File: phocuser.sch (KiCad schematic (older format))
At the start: 44 parts, among them J1 Conn_01x04_Male, J2 Conn_ARM_JTAG_SWD_10, J3 Conn_01x02_Male, J4 DX07S016JA1R1500, J5 Accessory 0, J6 Accessory 1, U1 HolyIot-18010, U2 TMC2130-LA, U3 FT231XQ

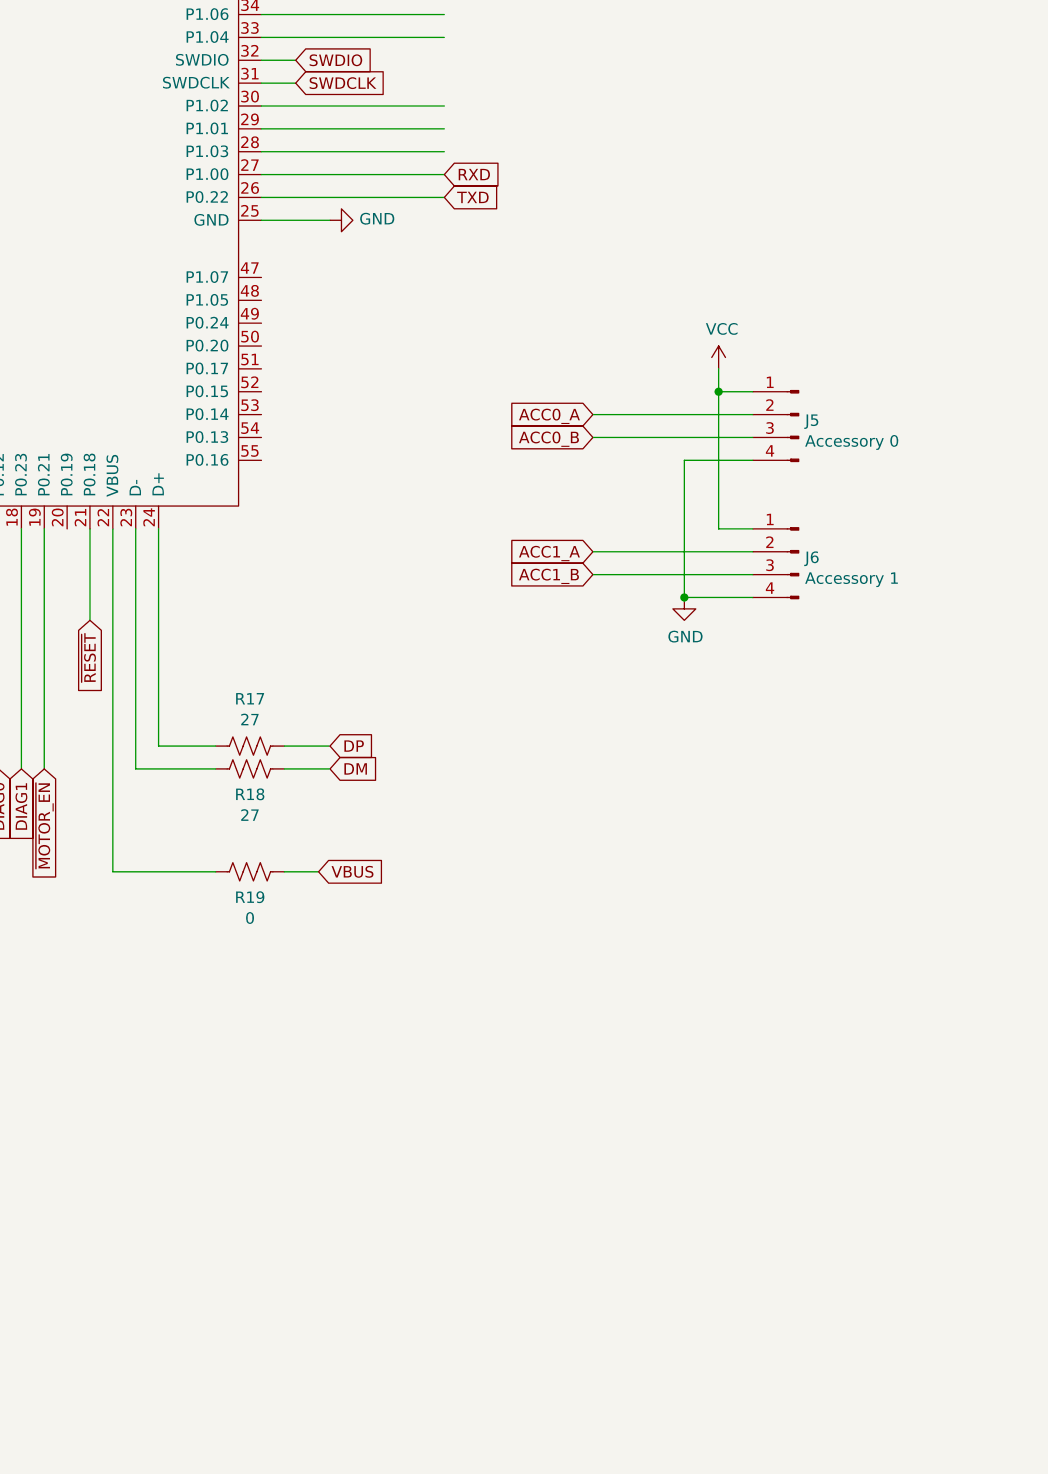
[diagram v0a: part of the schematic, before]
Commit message: layout complete
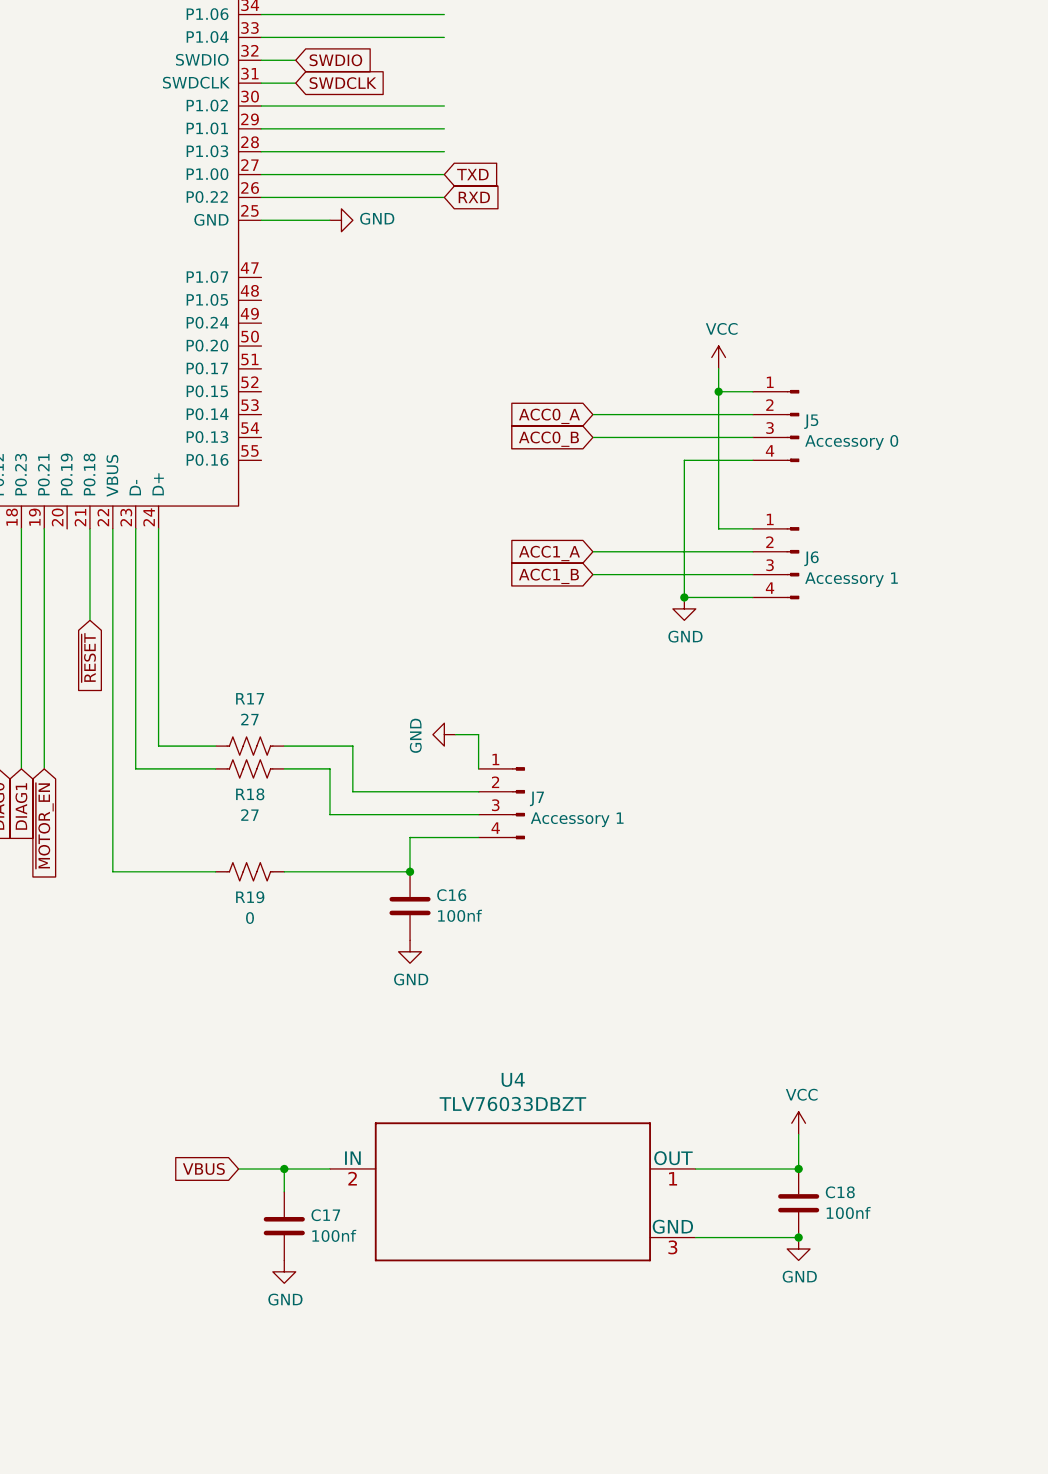
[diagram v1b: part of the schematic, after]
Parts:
- added C16, C17, C18: 100nf, Capacitor_SMD:C_0402_1005Metric, symbol Device:C
- added J7: Accessory 1, Connector_JST:JST_PH_B4B-PH-K_1x04_P2.00mm_Vertical, symbol Connector:Conn_01x04_Male
- added U4: TLV76033DBZT, footprints:TLV76033DBZT, symbol 2021-02-23_16-41-07:TLV76033DBZT
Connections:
- wire segments 191 -> 205
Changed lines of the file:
@@
 Wire Wire Line
 	4450 9450 4450 9600
+Text GLabel 6600 2400 2    50   Input ~ 0
+TXD
 Text GLabel 6600 2500 2    50   Input ~ 0
-TXD
-Text GLabel 6600 2400 2    50   Input ~ 0
 RXD
 $Comp
@@
 	0    1    1    0
 $EndComp
-Text GLabel 6100 4900 2    50   Input ~ 0
-DP
-Text GLabel 6100 5000 2    50   Input ~ 0
-DM
 Wire Wire Line
 	5350 3950 5350 4900
 Wire Wire Line
 	5350 4900 5600 4900
-Wire Wire Line
-	5900 4900 6100 4900
 Wire Wire Line
 	6100 5000 5900 5000
@@
 Wire Wire Line
 	5150 5450 5150 3950
-Text GLabel 6050 5450 2    50   Input ~ 0
-VBUS
-Wire Wire Line
-	6050 5450 5900 5450
 $Comp
 L Connector:Conn_01x04_Male J5
@@
 $EndComp
 Connection ~ 14350 1400
+$Comp
+L Connector:Conn_01x04_Male J7
+U 1 1 607FEF98
+P 6950 5100
+F 0 "J7" H 6922 5074 50  0000 R CNN
+F 1 "Accessory 1" H 6922 4983 50  0000 R CNN
+F 2 "Connector_JST:JST_PH_B4B-PH-K_1x04_P2.00mm_Vertical" H 6950 5100 50  0001 C CNN
+F 3 "~" H 6950 5100 50  0001 C CNN
+	1    6950 5100
+	-1   0    0    -1
+$EndComp
+Wire Wire Line
+	6450 5450 6450 5300
+Wire Wire Line
+	6450 5300 6750 5300
+Wire Wire Line
+	5900 5450 6450 5450
+$Comp
+L power:GND #PWR0123
+U 1 1 6084ADE6
+P 6650 4850
+F 0 "#PWR0123" H 6650 4600 50  0001 C CNN
+F 1 "GND" H 6655 4677 50  0000 C CNN
+F 2 "" H 6650 4850 50  0001 C CNN
+F 3 "" H 6650 4850 50  0001 C CNN
+	1    6650 4850
+	0    1    1    0
+$EndComp
+Wire Wire Line
+	6650 4850 6750 4850
+Wire Wire Line
+	6750 4850 6750 5000
+Wire Wire Line
+	6100 5000 6100 5200
+Wire Wire Line
+	6100 5200 6750 5200
+Wire Wire Line
+	6750 5100 6200 5100
+Wire Wire Line
+	6200 5100 6200 4900
+Wire Wire Line
+	5900 4900 6200 4900
+$Comp
+L Device:C C16
+U 1 1 6087547B
+P 6450 5600
+F 0 "C16" H 6565 5646 50  0000 L CNN
+F 1 "100nf" H 6565 5555 50  0000 L CNN
+F 2 "Capacitor_SMD:C_0402_1005Metric" H 6488 5450 50  0001 C CNN
+F 3 "~" H 6450 5600 50  0001 C CNN
+	1    6450 5600
+	1    0    0    -1
+$EndComp
+Connection ~ 6450 5450
+$Comp
+L power:GND #PWR0124
+U 1 1 60875FE1
+P 6450 5750
+F 0 "#PWR0124" H 6450 5500 50  0001 C CNN
+F 1 "GND" H 6455 5577 50  0000 C CNN
+F 2 "" H 6450 5750 50  0001 C CNN
+F 3 "" H 6450 5750 50  0001 C CNN
+	1    6450 5750
+	1    0    0    -1
+$EndComp
+$Comp
+L 2021-02-23_16-41-07:TLV76033DBZT U4
+U 1 1 608F0CB3
+P 6900 6850
+F 0 "U4" H 6900 7338 60  0000 C CNN
+F 1 "TLV76033DBZT" H 6900 7232 60  0000 C CNN
+F 2 "footprints:TLV76033DBZT" H 6900 6790 60  0001 C CNN
+F 3 "" H 6900 6850 60  0000 C CNN
+	1    6900 6850
+	1    0    0    -1
+$EndComp
+$Comp
+L Device:C C18
+U 1 1 608F9D14
+P 8150 6900
+F 0 "C18" H 8265 6946 50  0000 L CNN
+F 1 "100nf" H 8265 6855 50  0000 L CNN
+F 2 "Capacitor_SMD:C_0402_1005Metric" H 8188 6750 50  0001 C CNN
+F 3 "~" H 8150 6900 50  0001 C CNN
+	1    8150 6900
+	1    0    0    -1
+$EndComp
+$Comp
+L Device:C C17
+U 1 1 608FAADA
+P 5900 7000
+F 0 "C17" H 6015 7046 50  0000 L CNN
+F 1 "100nf" H 6015 6955 50  0000 L CNN
+F 2 "Capacitor_SMD:C_0402_1005Metric" H 5938 6850 50  0001 C CNN
+F 3 "~" H 5900 7000 50  0001 C CNN
+	1    5900 7000
+	1    0    0    -1
+$EndComp
+$Comp
+L power:GND #PWR0125
+U 1 1 608FBEA5
+P 5900 7150
+F 0 "#PWR0125" H 5900 6900 50  0001 C CNN
+F 1 "GND" H 5905 6977 50  0000 C CNN
+F 2 "" H 5900 7150 50  0001 C CNN
+F 3 "" H 5900 7150 50  0001 C CNN
+	1    5900 7150
+	1    0    0    -1
+$EndComp
+$Comp
+L power:GND #PWR0126
+U 1 1 608FD132
+P 8150 7050
+F 0 "#PWR0126" H 8150 6800 50  0001 C CNN
+F 1 "GND" H 8155 6877 50  0000 C CNN
+F 2 "" H 8150 7050 50  0001 C CNN
+F 3 "" H 8150 7050 50  0001 C CNN
+	1    8150 7050
+	1    0    0    -1
+$EndComp
+$Comp
+L power:VCC #PWR0137
+U 1 1 608FE384
+P 8150 6600
+F 0 "#PWR0137" H 8150 6450 50  0001 C CNN
+F 1 "VCC" H 8165 6773 50  0000 C CNN
+F 2 "" H 8150 6600 50  0001 C CNN
+F 3 "" H 8150 6600 50  0001 C CNN
+	1    8150 6600
+	1    0    0    -1
+$EndComp
+Wire Wire Line
+	5900 6850 5900 6750
+Wire Wire Line
+	5900 6750 6100 6750
+Wire Wire Line
+	7700 6750 8150 6750
+Wire Wire Line
+	8150 6750 8150 6600
+Connection ~ 8150 6750
+Wire Wire Line
+	7700 7050 8150 7050
+Connection ~ 8150 7050
+Text GLabel 5700 6750 0    50   Input ~ 0
+VBUS
+Wire Wire Line
+	5900 6750 5700 6750
+Connection ~ 5900 6750
 $EndSCHEMATC
